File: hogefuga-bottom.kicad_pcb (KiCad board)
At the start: 2 copper layers, 95.2 x 97.6 mm, 6 parts

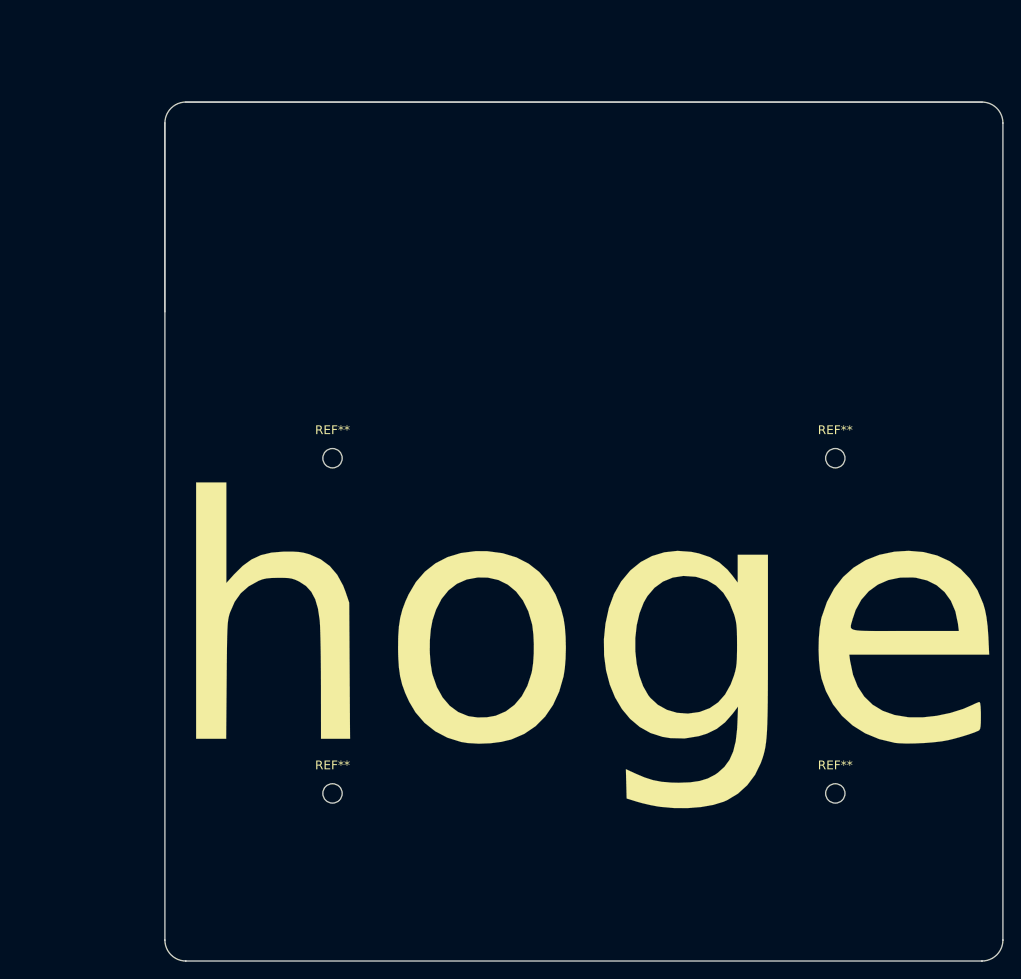
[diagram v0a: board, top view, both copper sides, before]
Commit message: rev0.2
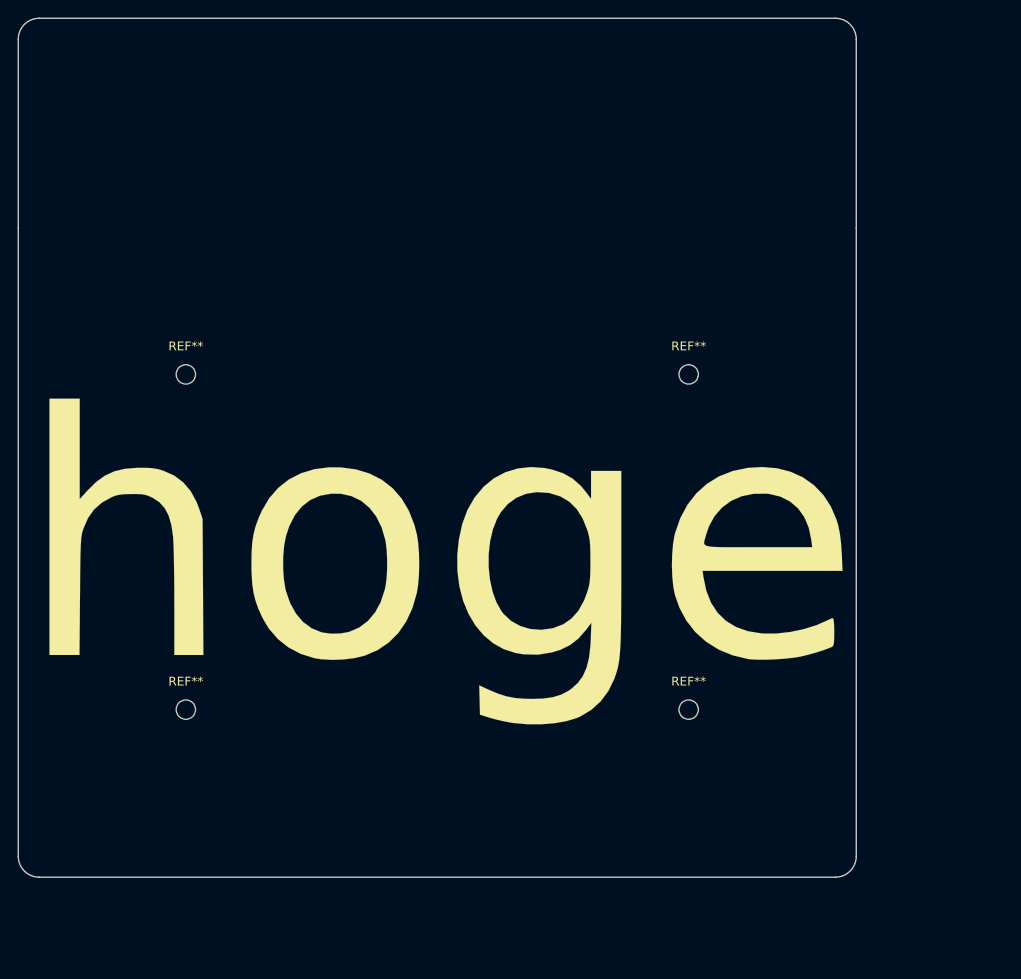
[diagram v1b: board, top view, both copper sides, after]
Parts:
- removed the REF** at (90.5, 126.2)
- removed the REF** at (147.6, 88.1)
- removed the REF** at (90.5, 88.1)
- removed the REF** at (147.6, 126.2)
- added REF**: MountingHole_2.2mm_M2, MountingHole:MountingHole_2.2mm_M2, F.Cu at (131.0, 78.6)
- added REF**: MountingHole_2.2mm_M2, MountingHole:MountingHole_2.2mm_M2, F.Cu at (131.0, 116.7)
- added REF**: MountingHole_2.2mm_M2, MountingHole:MountingHole_2.2mm_M2, F.Cu at (73.8, 116.7)
- added REF**: MountingHole_2.2mm_M2, MountingHole:MountingHole_2.2mm_M2, F.Cu at (73.8, 78.6)
- moved G*** 19.2 mm to (102.4, 100.0) (x2)
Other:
- board size 95.2 x 97.6 mm -> 95.3 x 97.6 mm
